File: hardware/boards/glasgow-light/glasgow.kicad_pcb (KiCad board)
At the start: 2 copper layers, 90.2 x 20.2 mm, 171 parts, among them J1 USB_C_USB2.0, J2 IDC-Header_2x5_P2.54mm, J3 IDC-Header_2x5_P2.54mm, U1 LM358_DFN, U10 SN74LVC1T45DCKR, U11 SN74LVC1T45DCKR, U12 INA180A2, U15 TPD3S014, U16 SN74LVC1T45DCKR, U17 SN74LVC1T45DCKR, U18 SN74LVC1T45DCKR, U19 PCA6408APW, U2 GD32VF103T, U31 TPS73101DBV, U36 TLV73312PQDRVR, U4 SN74LVC1T45DCKR, U5 ICE40UP5K-SG48ITR, U6 SN74LVC1T45DCKR, U8 TLV75533PDRVR, U9 SN74LVC1T45DCKR, Y1 8M

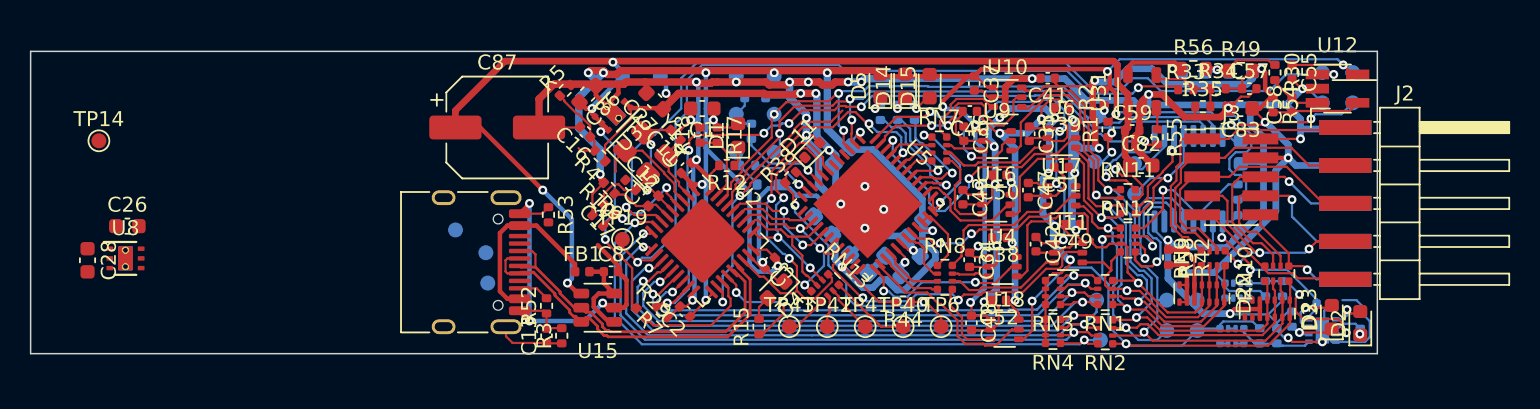
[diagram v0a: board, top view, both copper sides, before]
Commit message: optimize
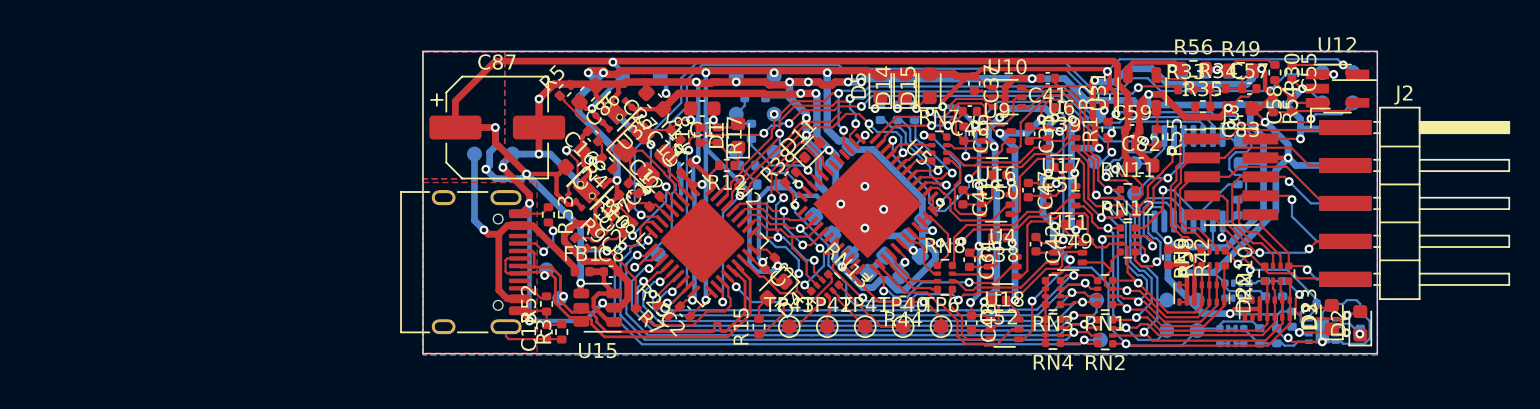
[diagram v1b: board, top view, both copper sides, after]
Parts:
- TP14, TP19: moved to B.Cu
- moved C28 34.6 mm to (122.3, 45.3), turned to 225 degrees
- moved U8 31.2 mm to (121.2, 43.2), turned to 225 degrees
- moved C26 30.2 mm to (120.3, 41.1), turned to 225 degrees
- moved TP14 27.7 mm to (116.2, 40.8)
- moved TP13 5.24 mm to (113.7, 40.8)
- moved TP16 4.93 mm to (119.4, 50.4)
- moved TP15 4.22 mm to (118.5, 48.5)
- moved TP19 2.62 mm to (126.0, 47.5)
- moved R9 1.90 mm to (120.8, 46.7)
- moved C17 1.78 mm to (124.0, 45.7), turned to 45 degrees
- moved R10 1.31 mm to (123.7, 43.9)
- moved R4 0.70 mm to (122.6, 41.4)
- moved C16 0.60 mm to (121.6, 39.6)
- moved C12 0.30 mm to (124.3, 43.1)
- moved C13 0.25 mm to (118.5, 52.7)
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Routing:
- net GND: track 367.1 -> 392.5 mm, vias 39 -> 42
- net +5V: track 91.2 -> 98.9 mm, vias 6 -> 7
- net /IO_Banks/VIOA: track 134.9 -> 127.6 mm
- net /xVBUS: track 12.2 -> 18.6 mm, vias 0 -> 1
- net Net-(C16-Pad1): track 5.87 -> 11.8 mm, vias 0 -> 2
- net /CC1: track 0.00 -> 4.19 mm, vias 0 -> 2
- net /USB_N: track 22.8 -> 25.7 mm, vias 0 -> 1
- net /NRST: track 7.06 -> 9.24 mm
- net /USB_P: track 24.8 -> 26.5 mm, vias 0 -> 1
- net +1V2: track 39.9 -> 41.1 mm
- net /VDDA: track 4.11 -> 3.01 mm
- net +3V3: track 240.7 -> 239.7 mm
- net VIO_CURRENT: track 61.4 -> 60.4 mm
- net /XTALIN: track 7.30 -> 7.99 mm
- net VIO_DAC: track 51.9 -> 51.3 mm
- added copper zone on B.Cu, net +5V
- added copper zone on F.Cu, net +5V
- added copper zone on F.Cu, net /SHLD
- added copper zone on B.Cu, net GND
- added copper zone on F.Cu, net GND
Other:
- board size 90.2 x 20.2 mm -> 63.9 x 20.2 mm
